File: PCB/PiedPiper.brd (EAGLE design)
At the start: 67.3 x 96.2 mm, 27 parts

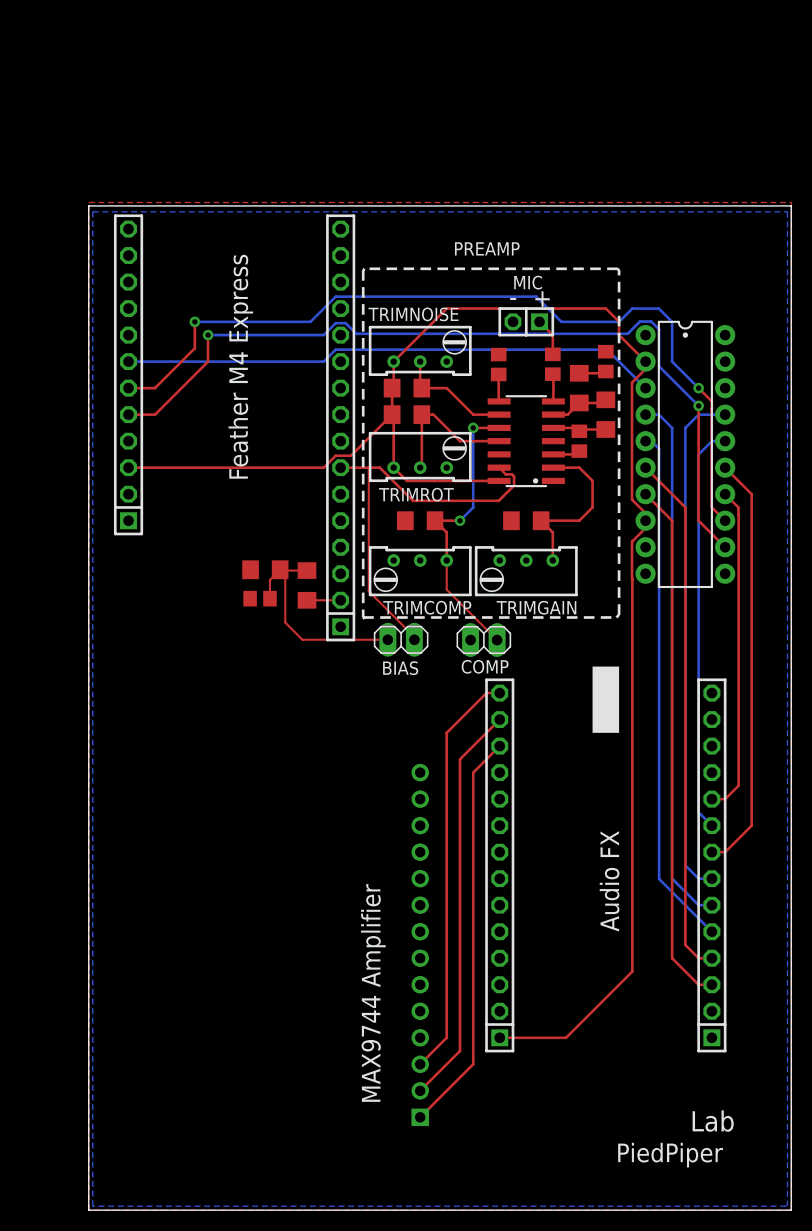
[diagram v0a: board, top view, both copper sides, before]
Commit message: Added updated PCB
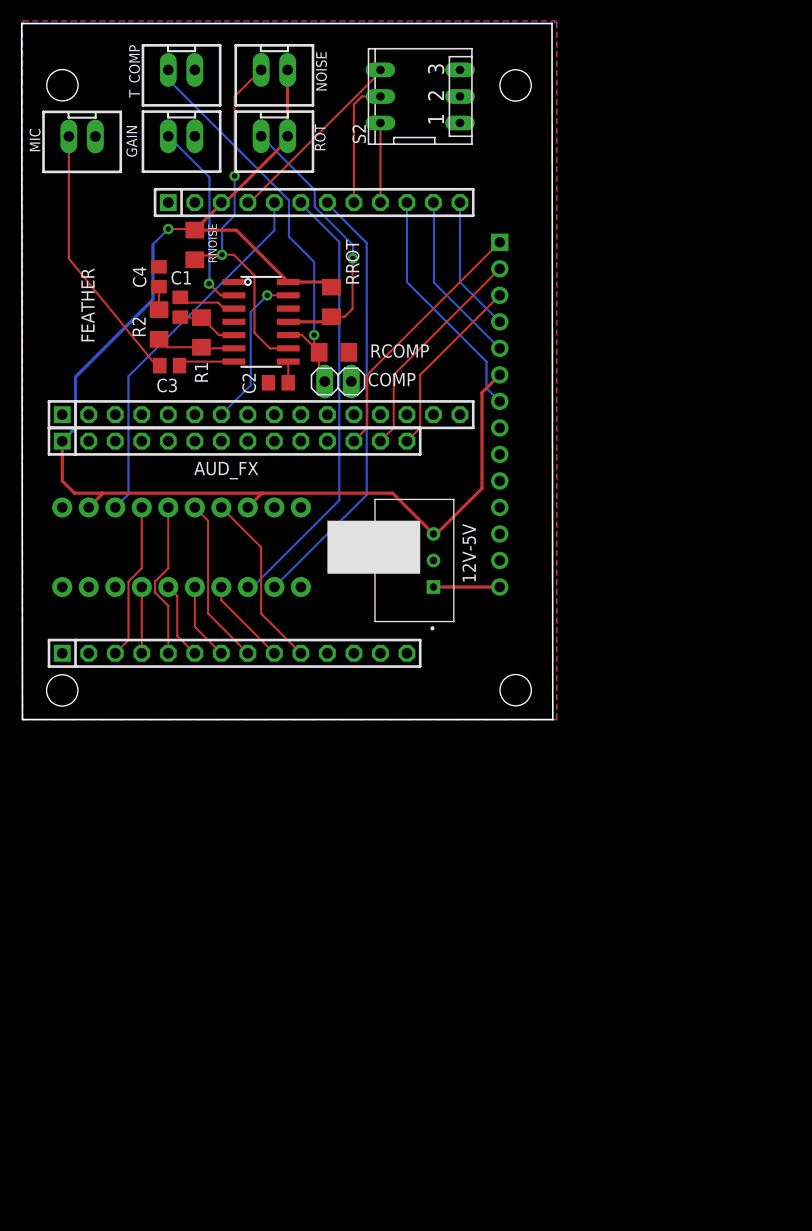
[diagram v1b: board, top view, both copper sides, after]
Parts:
- removed BIAS: (no value), pinhead:1X02
- removed C5: 1u, rcl:C0805
- removed MAX97_INPUT: (no value), microbuilder:1X14_ROUND70
- removed RGAIN: (no value), rcl:R1206
- removed R_DIVIDE1, R_DIVIDE2: 10k, rcl:R1206
- removed TRIMCOMP, TRIMGAIN, TRIMNOISE, TRIMROT: (no value), rcl:RTRIM64W
- added 12V-5V: TSR_1-2450, TSR_1-2450:CONV_TSR_1-2450
- added GAIN, NOISE, ROT, T_COMP: JST-XH-02-PIN-LONG-PAD, Rembrandt Electronics - JST XH Connectors v1-0:JST-XH-02-PACKAGE-LONG-PAD
- added MAX97_AMPLIFIER: (no value), microbuilder:1X14_ROUND70
- added S2: (no value), switch-dil:DP-03
- MIC: value (none) -> JST-XH-02-PIN-LONG-PAD; device pinhead:1X02 -> Rembrandt Electronics - JST XH Connectors v1-0:JST-XH-02-PACKAGE-LONG-PAD
- moved AUD_PINS 50.0 mm to (17.8, 54.6), turned to 0 degrees
- moved SHIFT_REGISTER 49.1 mm to (12.7, 64.8), flipped to the bottom, turned to 180 degrees
- moved AUD_FX 47.9 mm to (17.8, 74.9), turned to 0 degrees
- moved MIC 46.1 mm to (3.17, 104.1)
- moved C4 43.6 mm to (10.5, 90.7)
- moved R2 40.7 mm to (10.5, 86.1)
- moved C1 40.3 mm to (12.6, 87.8), turned to 90 degrees
- moved R1 39.5 mm to (14.6, 85.3), turned to 270 degrees
- moved C3 36.7 mm to (11.6, 82.2), turned to 0 degrees
- moved COMP 28.4 mm to (27.7, 80.6), turned to 0 degrees
- moved PREAMP 27.9 mm to (20.3, 86.4), turned to 270 degrees
- moved RNOISE 24.5 mm to (14.0, 93.7), turned to 270 degrees
- moved FEATHER2 24.3 mm to (25.4, 97.8), turned to 0 degrees
- moved C2 21.2 mm to (22.0, 80.5), turned to 180 degrees
- moved RCOMP 18.1 mm to (27.3, 83.4), turned to 0 degrees
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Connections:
- removed net 3V: FEATHER.2, R_DIVIDE1.1
- removed net BIAS: BIAS.1, C5.1, R_DIVIDE1.2, R_DIVIDE2.1
- removed net SCL_5V0: MAX97_INPUT.5
- removed net SDA_5V0: MAX97_INPUT.4
- removed net VDDIO: MAX97_INPUT.6
- new net N$1: FEATHER2.8, S2.5
- new net N$3: FEATHER2.9, S2.6
- new net N$4: FEATHER2.4, S2.4
- new net SCL: FEATHER2.11, MAX97_AMPLIFIER.5
- new net SDA: FEATHER2.12, MAX97_AMPLIFIER.4
- net A2: no longer BIAS.2
- net ADDR1_5V: now also MAX97_AMPLIFIER.11; no longer MAX97_INPUT.11
- net ADDR2_5V: now also MAX97_AMPLIFIER.12; no longer MAX97_INPUT.12
- net AGND: now also MAX97_AMPLIFIER.3; no longer MAX97_INPUT.3
- net AUD1: now also SHIFT_REGISTER.4; no longer SHIFT_REGISTER.7
- net AUD2: now also SHIFT_REGISTER.17; no longer SHIFT_REGISTER.6
- net AUD4: now also SHIFT_REGISTER.16; no longer SHIFT_REGISTER.4
- net AUD5: now also SHIFT_REGISTER.15; no longer SHIFT_REGISTER.17
- net AUD6: now also SHIFT_REGISTER.6; no longer SHIFT_REGISTER.15
- net AUD7: now also SHIFT_REGISTER.14; no longer SHIFT_REGISTER.16
- net AUD8: now also SHIFT_REGISTER.7; no longer SHIFT_REGISTER.14
- net AUDIOIN: now also MIC.2; no longer MIC.1
- net CLOCK: now also FEATHER2.6, SHIFT_REGISTER.13; no longer FEATHER2.5, SHIFT_REGISTER.12
- net COMP: now also T_COMP.2; no longer TRIMCOMP.1
- net GAIN: now also GAIN.2; no longer RGAIN.2, TRIMGAIN.1
- net GND: now also 12V-5V.2, GAIN.1, MAX97_AMPLIFIER.13, MIC.1, S2.1, S2.2, S2.3, T_COMP.1; no longer C5.2, MAX97_INPUT.13, MIC.2, RGAIN.1, R_DIVIDE2.2, TRIMCOMP.2, TRIMGAIN.2
- net LATCH: now also FEATHER2.7, SHIFT_REGISTER.12; no longer FEATHER2.6, SHIFT_REGISTER.13
- net LAUDIO: now also MAX97_AMPLIFIER.2; no longer MAX97_INPUT.2
- net MUTE_INV: now also MAX97_AMPLIFIER.8; no longer MAX97_INPUT.8
- net NOISE: now also NOISE.2; no longer TRIMNOISE.2
- net RAUDIO: now also MAX97_AMPLIFIER.1; no longer MAX97_INPUT.1
- net ROT: now also ROT.2; no longer TRIMROT.2
- net SER_IN: now also FEATHER2.5; no longer FEATHER2.7
- net SHDN_5V: now also FEATHER2.10, MAX97_AMPLIFIER.7; no longer MAX97_INPUT.7
- net SYNCOUT: now also MAX97_AMPLIFIER.9; no longer MAX97_INPUT.9
- net SYNC_5V: now also MAX97_AMPLIFIER.10; no longer MAX97_INPUT.10
- net USB: now also 12V-5V.3, MAX97_AMPLIFIER.6, NOISE.1, ROT.1; no longer TRIMNOISE.1, TRIMROT.1
- net VDD: now also 12V-5V.1, MAX97_AMPLIFIER.14; no longer MAX97_INPUT.14
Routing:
- net AUD2: track 50.4 -> 6.35 mm
- net AUD4: track 51.1 -> 7.41 mm
- net AUD5: track 49.3 -> 7.40 mm
- net CLOCK: track 80.6 -> 42.3 mm, vias 2 -> 0
- net LATCH: track 80.4 -> 42.1 mm, vias 2 -> 0
- net AUD1: track 50.4 -> 15.0 mm
- net AUD3: track 49.9 -> 15.0 mm
- net AUD7: track 39.2 -> 8.45 mm
- net USB: track 152.9 -> 125.0 mm, vias 0 -> 1
- net NOISE: track 11.1 -> 35.6 mm, vias 0 -> 2
- net A2: track 39.5 -> 15.3 mm, vias 0 -> 1
- net AUD6: track 40.2 -> 16.1 mm
- net SHDN_5V: track 0.00 -> 22.7 mm
- net AUDIOIN: track 3.64 -> 25.8 mm
- net AGND: track 39.5 -> 17.7 mm
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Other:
- board size 67.3 x 96.2 mm -> 50.9 x 66.7 mm
- board text removed: "+"
- board text removed: "-"
- board text removed: "Audio FX"
- board text removed: "Feather M4 Express"
- board text removed: "Lab"
- board text removed: "MAX9744 Amplifier"
- board text removed: "PiedPiper"
